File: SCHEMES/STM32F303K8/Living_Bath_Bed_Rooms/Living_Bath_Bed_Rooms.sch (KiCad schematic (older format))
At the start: 24 parts, among them M1 Ceiling_Fan, Q1 Q_NMOS_DGS, Q1 Q_NPN_CBE, U1 STM32F303K8Tx

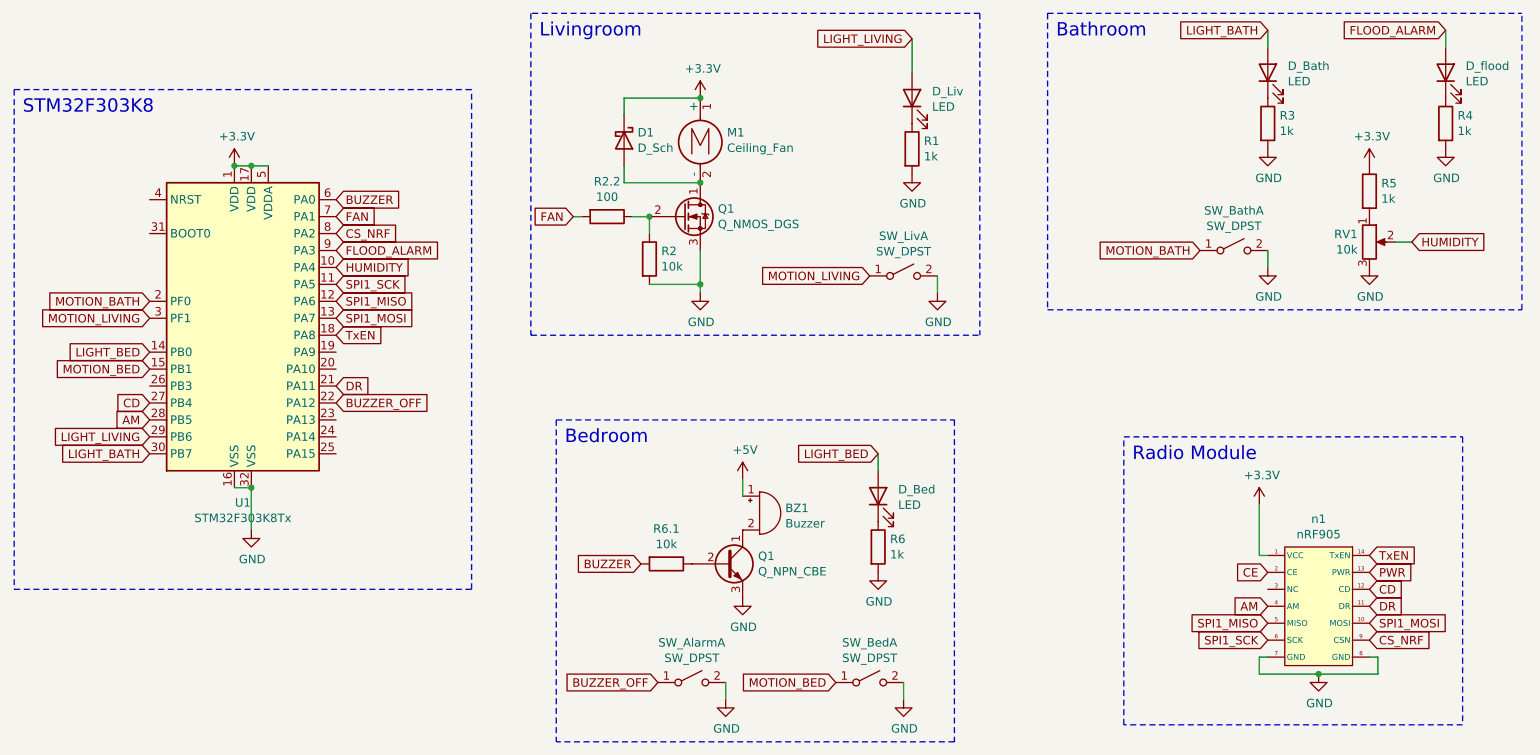
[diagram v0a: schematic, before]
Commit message: Schema corrections
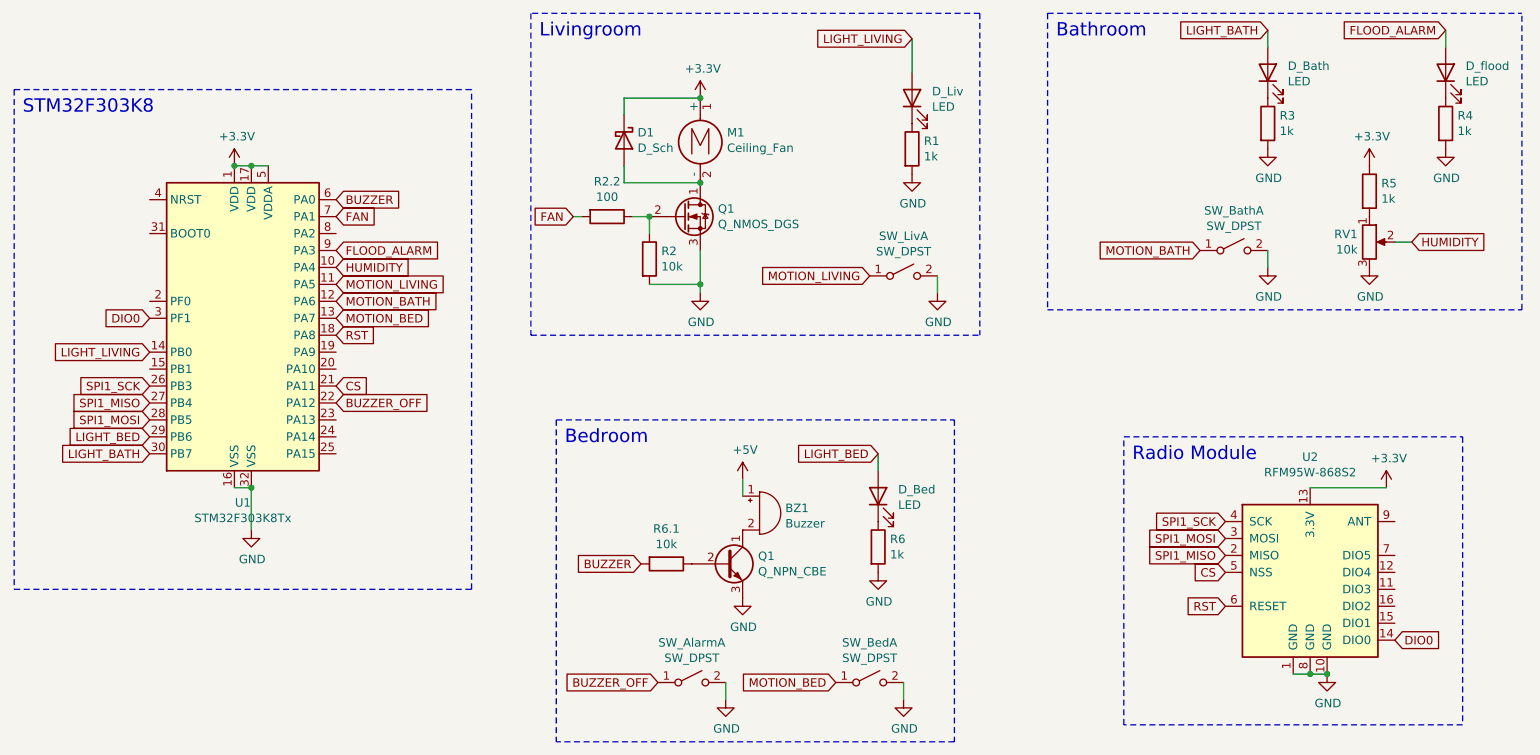
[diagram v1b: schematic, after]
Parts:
- removed n1: nRF905, symbol Living_Bath_Bed_Rooms-rescue:nRF905-nrf_custom2
- added U2: RFM95W-868S2, symbol RF_Module:RFM95W-868S2
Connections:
- net AM is gone; now on net SPI1_MOSI: U1.28 (PB5)
- net CD is gone; now on net SPI1_MISO: U1.27 (PB4)
- net +3V3: now also U2.13 (3.3V)
- net GND: now also U2.1 (GND), U2.10 (GND), U2.8 (GND)
- net LIGHT_BED: now also U1.29 (PB6); no longer U1.14 (PB0)
- net LIGHT_LIVING: now also U1.14 (PB0); no longer U1.29 (PB6)
- net MOTION_BATH: now also U1.12 (PA6); no longer U1.2 (PF0)
- net MOTION_BED: now also U1.13 (PA7); no longer U1.15 (PB1)
- net MOTION_LIVING: now also U1.11 (PA5); no longer U1.3 (PF1)
- net SPI1_MISO: now also U2.2 (MISO); no longer U1.12 (PA6)
- net SPI1_MOSI: now also U2.3 (MOSI); no longer U1.13 (PA7)
- net SPI1_SCK: now also U1.26 (PB3), U2.4 (SCK); no longer U1.11 (PA5)
- net CS_NRF: no longer names the net of U1.8 (PA2)
- net DR renamed CS
- net CS: now also U2.5 (NSS)
- net TxEN renamed RST
- net RST: now also U2.6 (RESET)
- new net DIO0: U1.3 (PF1), U2.14 (DIO0)
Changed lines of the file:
@@
 Text GLabel 3250 2250 2    50   Input ~ 0
 BUZZER
-Text GLabel 3250 2450 2    50   Input ~ 0
-CS_NRF
 Text GLabel 3250 2550 2    50   Input ~ 0
 FLOOD_ALARM
 Text GLabel 3250 2650 2    50   Input ~ 0
 HUMIDITY
-Text GLabel 3250 2750 2    50   Input ~ 0
+Text GLabel 2150 3350 0    50   Input ~ 0
 SPI1_SCK
-Text GLabel 3250 2850 2    50   Input ~ 0
+Text GLabel 2150 3450 0    50   Input ~ 0
 SPI1_MISO
-Text GLabel 3250 2950 2    50   Input ~ 0
+Text GLabel 2150 3550 0    50   Input ~ 0
 SPI1_MOSI
 Text GLabel 3250 3050 2    50   Input ~ 0
-TxEN
-Text GLabel 3250 3350 2    50   Input ~ 0
-DR
+RST
 Text GLabel 3250 3450 2    50   Input ~ 0
 BUZZER_OFF
-Text GLabel 2150 2850 0    50   Input ~ 0
+Text GLabel 3250 2850 2    50   Input ~ 0
 MOTION_BATH
+Text GLabel 3250 2750 2    50   Input ~ 0
+MOTION_LIVING
+Text GLabel 3250 2950 2    50   Input ~ 0
+MOTION_BED
+Text GLabel 3250 3350 2    50   Input ~ 0
+CS
 Text GLabel 2150 2950 0    50   Input ~ 0
-MOTION_LIVING
+DIO0
 Text GLabel 2150 3150 0    50   Input ~ 0
-LIGHT_BED
-Text GLabel 2150 3250 0    50   Input ~ 0
-MOTION_BED
-Text GLabel 2150 3450 0    50   Input ~ 0
-CD
-Text GLabel 2150 3550 0    50   Input ~ 0
-AM
-Text GLabel 2150 3650 0    50   Input ~ 0
 LIGHT_LIVING
 Text GLabel 2150 3750 0    50   Input ~ 0
@@
 Wire Notes Line
 	4550 3550 4550 5450
-$Comp
-L Living_Bath_Bed_Rooms-rescue:nRF905-nrf_custom2 n1
-U 1 1 60EC89FE
-P 9050 4300
-F 0 "n1" H 9050 4465 50  0000 C CNN
-F 1 "nRF905" H 9050 4374 50  0000 C CNN
-F 2 "" H 9050 4400 50  0001 C CNN
-F 3 "" H 9050 4400 50  0001 C CNN
-	1    9050 4300
-	1    0    0    -1
-$EndComp
-$Comp
-L power:GND #PWR?
-U 1 1 60ECDF57
-P 9050 5050
-F 0 "#PWR?" H 9050 4800 50  0001 C CNN
-F 1 "GND" H 9055 4877 50  0000 C CNN
-F 2 "" H 9050 5050 50  0001 C CNN
-F 3 "" H 9050 5050 50  0001 C CNN
-	1    9050 5050
-	1    0    0    -1
-$EndComp
-Wire Wire Line
-	8750 4950 8700 4950
-Wire Wire Line
-	8700 4950 8700 5050
-Wire Wire Line
-	8700 5050 9050 5050
-Wire Wire Line
-	9350 4950 9400 4950
-Wire Wire Line
-	9400 4950 9400 5050
-Wire Wire Line
-	9400 5050 9050 5050
-Connection ~ 9050 5050
-$Comp
-L power:+3.3V #PWR?
-U 1 1 60ECF864
-P 8700 4050
-F 0 "#PWR?" H 8700 3900 50  0001 C CNN
-F 1 "+3.3V" H 8715 4223 50  0000 C CNN
-F 2 "" H 8700 4050 50  0001 C CNN
-F 3 "" H 8700 4050 50  0001 C CNN
-	1    8700 4050
-	1    0    0    -1
-$EndComp
-Wire Wire Line
-	8700 4350 8750 4350
-Text GLabel 8750 4850 0    50   Input ~ 0
-SPI1_SCK
-Text GLabel 8750 4750 0    50   Input ~ 0
-SPI1_MISO
-Text GLabel 9350 4750 2    50   Input ~ 0
-SPI1_MOSI
-Text GLabel 9350 4550 2    50   Input ~ 0
-CD
-Text GLabel 8750 4650 0    50   Input ~ 0
-AM
-Text GLabel 9350 4850 2    50   Input ~ 0
-CS_NRF
-Text GLabel 9350 4350 2    50   Input ~ 0
-TxEN
-Text GLabel 9350 4650 2    50   Input ~ 0
-DR
 Text Notes 7950 3800 0    79   ~ 0
 Radio Module\n
@@
 Text Notes 1400 1750 0    79   ~ 0
 STM32F303K8
-Wire Notes Line
-	1350 1600 1350 4550
 Wire Notes Line
 	1350 4550 4050 4550
@@
 	0    1    1    0
 $EndComp
-Wire Wire Line
-	8700 4050 8700 4350
-Text GLabel 8750 4450 0    50   Input ~ 0
-CE
-Text GLabel 9350 4450 2    50   Input ~ 0
-PWR
+Wire Notes Line
+	1350 1600 1350 4550
+Text GLabel 2150 3650 0    50   Input ~ 0
+LIGHT_BED
+$Comp
+L RF_Module:RFM95W-868S2 U2
+U 1 1 61830682
+P 9000 4450
+F 0 "U2" H 9000 5131 50  0000 C CNN
+F 1 "RFM95W-868S2" H 9000 5040 50  0000 C CNN
+F 2 "" H 5700 6100 50  0001 C CNN
+F 3 "https://www.hoperf.com/data/upload/portal/20181127/5bfcbea20e9ef.pdf" H 5700 6100 50  0001 C CNN
+	1    9000 4450
+	1    0    0    -1
+$EndComp
+$Comp
+L power:+3.3V #PWR?
+U 1 1 60ECF864
+P 9450 3950
+F 0 "#PWR?" H 9450 3800 50  0001 C CNN
+F 1 "+3.3V" H 9465 4123 50  0000 C CNN
+F 2 "" H 9450 3950 50  0001 C CNN
+F 3 "" H 9450 3950 50  0001 C CNN
+	1    9450 3950
+	1    0    0    -1
+$EndComp
+Text GLabel 8500 4150 0    50   Input ~ 0
+SPI1_SCK
+Text GLabel 8500 4350 0    50   Input ~ 0
+SPI1_MISO
+Text GLabel 8500 4250 0    50   Input ~ 0
+SPI1_MOSI
+Text GLabel 8500 4650 0    50   Input ~ 0
+RST
+Text GLabel 8500 4450 0    50   Input ~ 0
+CS
+$Comp
+L power:GND #PWR?
+U 1 1 6183A380
+P 9100 5050
+F 0 "#PWR?" H 9100 4800 50  0001 C CNN
+F 1 "GND" H 9105 4877 50  0000 C CNN
+F 2 "" H 9100 5050 50  0001 C CNN
+F 3 "" H 9100 5050 50  0001 C CNN
+	1    9100 5050
+	1    0    0    -1
+$EndComp
+Wire Wire Line
+	9450 3950 9000 3950
+Wire Wire Line
+	8900 5050 9000 5050
+Wire Wire Line
+	9000 5050 9100 5050
+Connection ~ 9000 5050
+Connection ~ 9100 5050
+Text GLabel 9500 4850 2    50   Input ~ 0
+DIO0
 $EndSCHEMATC

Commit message: Final version
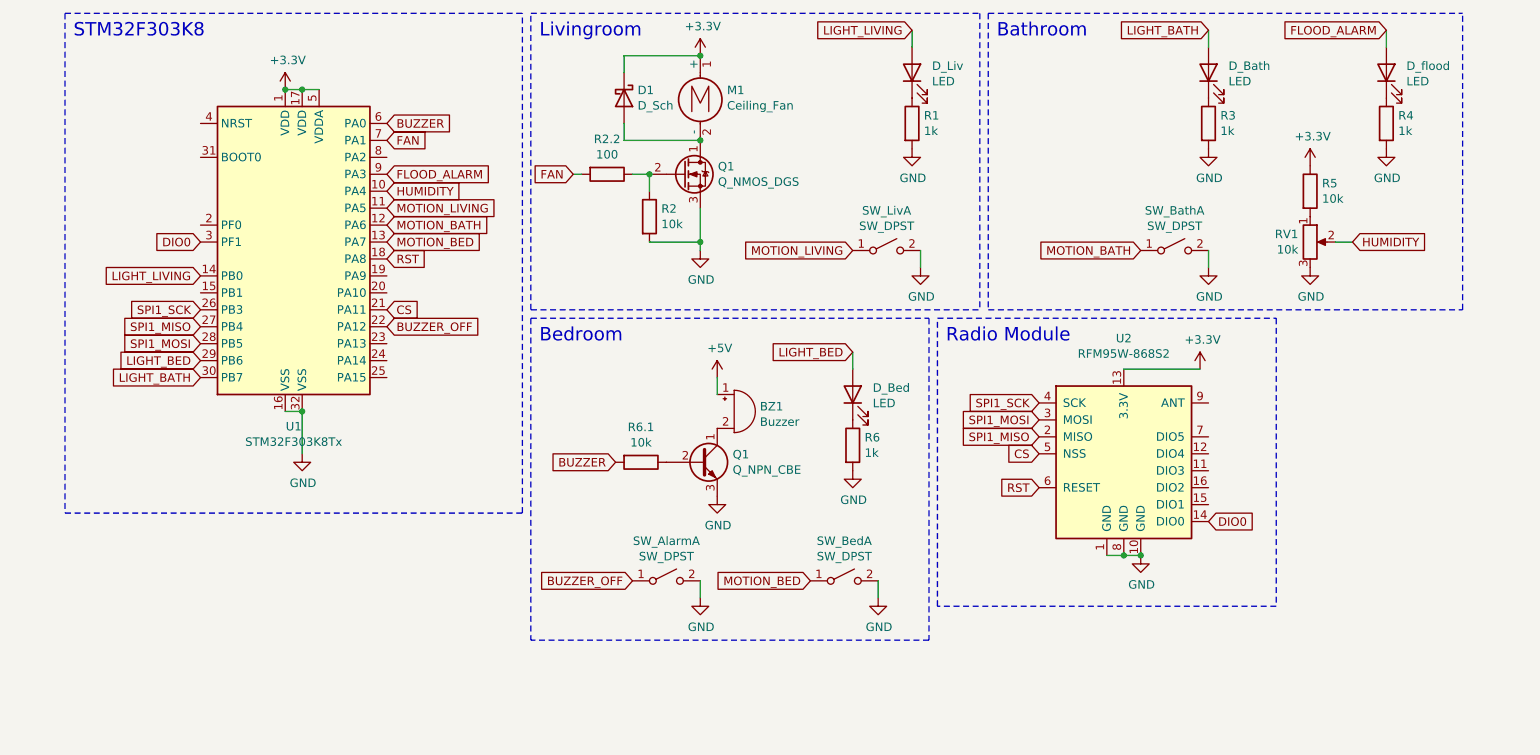
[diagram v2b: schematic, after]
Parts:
- R5: value 1k -> 10k
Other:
- moved on the sheet: BZ1, D1, D_Bath, D_Bed, D_Liv, D_flood, M1, Q1, R1, R2, R2.2, R3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
